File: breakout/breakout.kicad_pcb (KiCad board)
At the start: 2 copper layers, 19.3 x 44.5 mm, 2 parts, among them J1 Conn_01x15, J2 Conn_01x15

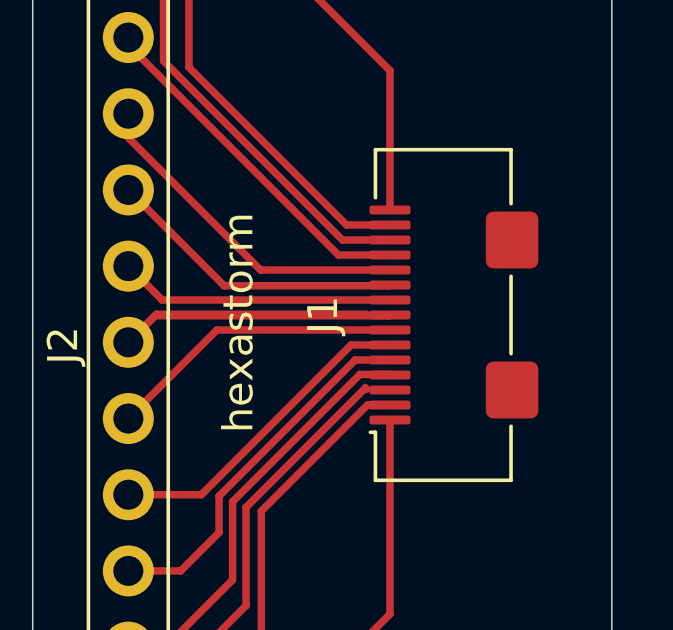
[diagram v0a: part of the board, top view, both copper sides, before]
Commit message: updated bom
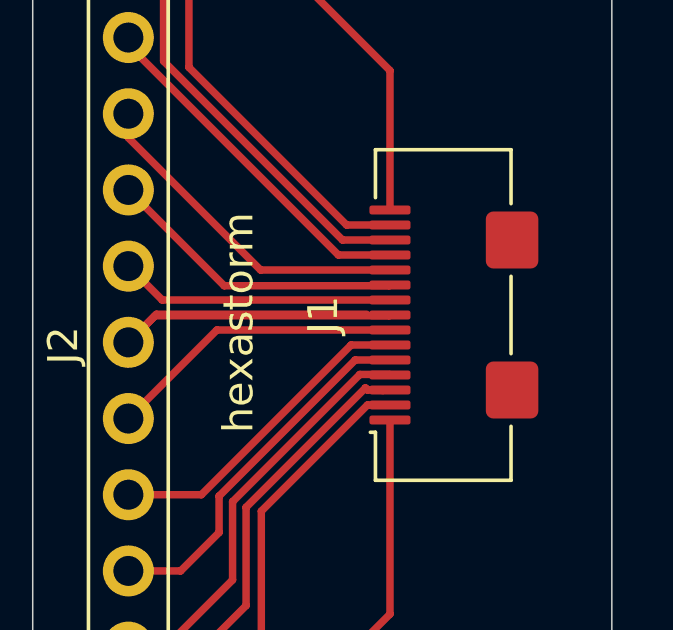
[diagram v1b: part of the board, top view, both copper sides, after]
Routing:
- net Net-(J1-Pad3): track 14.5 -> 15.1 mm
